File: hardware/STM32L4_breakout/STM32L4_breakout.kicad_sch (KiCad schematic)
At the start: 64 parts, among them J1 12V IN, J10 GPIO, J11 SPI1, J12 USART1, J13 USART3, J14 UART4, J15 3.3V, J16 5V, J17 12V, J2 SWD, J3 Conn_01x08, J4 Conn_01x06, J5 Conn_01x10, J6 Conn_01x08, J7 I2C1, J8 I2C2, J9 I2C3, SW1 SW_SPDT, U1 LD1117S50TR_SOT223, U2 LD3985M33R_SOT23, U3 LD1117S33TR_SOT223, U4 STM32L476RGTx, X1 NX3215SA-32.768K

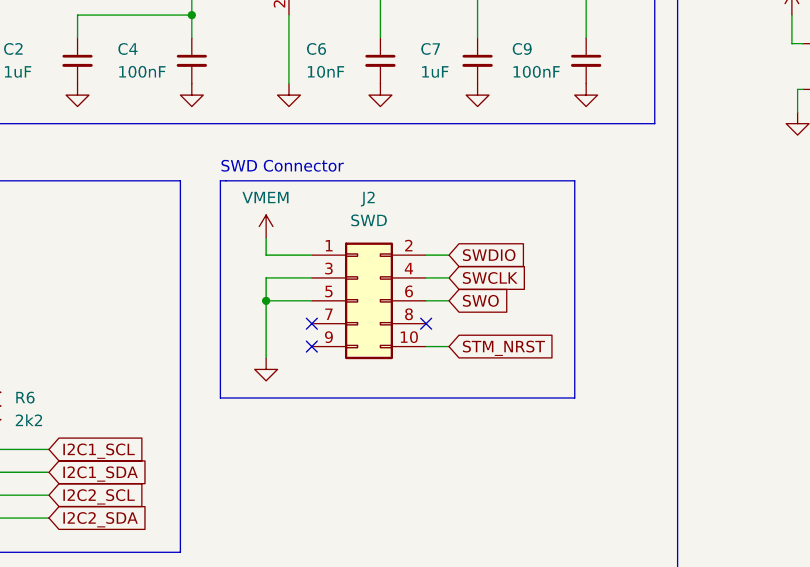
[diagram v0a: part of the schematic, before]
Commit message: breakout board PCB layout WIP
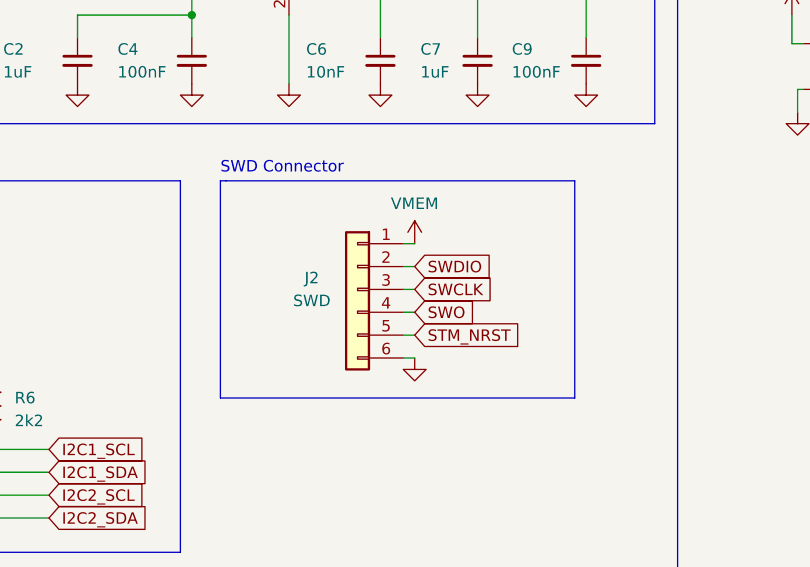
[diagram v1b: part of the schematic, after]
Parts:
- removed J2: SWD, Connector_PinHeader_2.54mm:PinHeader_2x05_P2.54mm_Vertical, symbol Connector_Generic:Conn_02x05_Odd_Even
- added J2: SWD, Connector_PinHeader_2.54mm:PinHeader_1x06_P2.54mm_Vertical, symbol Connector_Generic:Conn_01x06
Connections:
- net GND: now also J2.6 (Pin_6)
- net STM_NRST: now also J2.5 (Pin_5)
- net SWCLK: now also J2.3 (Pin_3)
- net SWDIO: now also J2.2 (Pin_2)
- net SWO: now also J2.4 (Pin_4)
- net VMEM: now also J2.1 (Pin_1)
- no-connect marks 33 -> 30

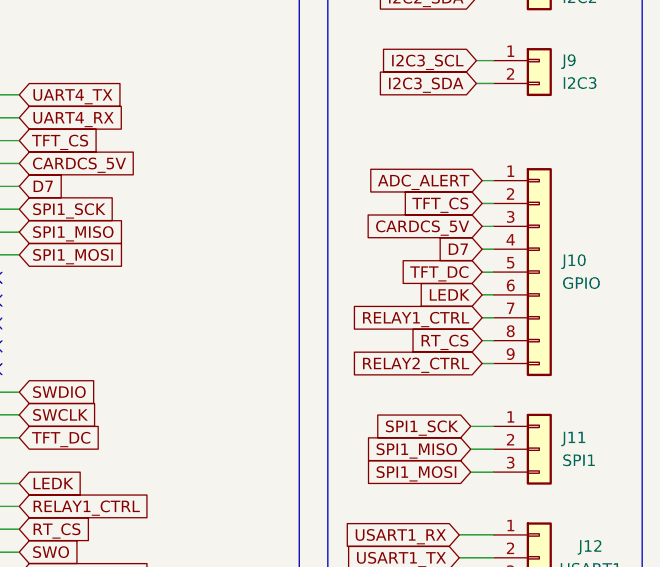
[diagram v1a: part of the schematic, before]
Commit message: breakout board PCB layout WIP
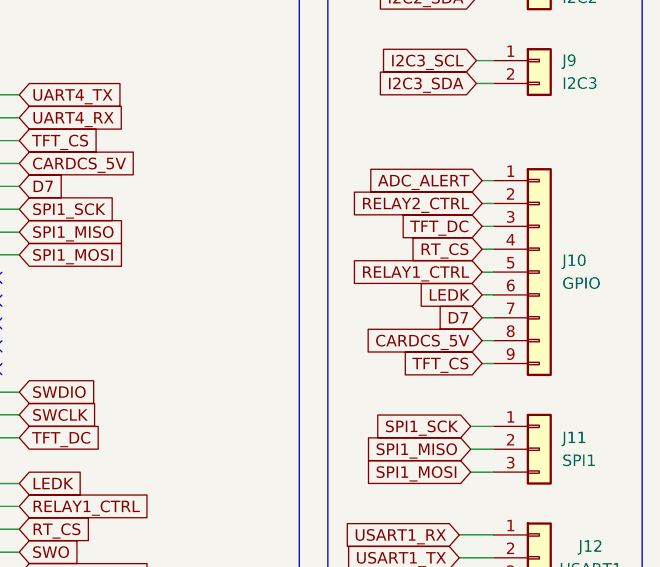
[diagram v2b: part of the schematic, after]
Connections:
- net CARDCS_5V: now also J10.8 (Pin_8); no longer J10.3 (Pin_3)
- net D7: now also J10.7 (Pin_7); no longer J10.4 (Pin_4)
- net RELAY1_CTRL: now also J10.5 (Pin_5); no longer J10.7 (Pin_7)
- net RELAY2_CTRL: now also J10.2 (Pin_2); no longer J10.9 (Pin_9)
- net RT_CS: now also J10.4 (Pin_4); no longer J10.8 (Pin_8)
- net TFT_CS: now also J10.9 (Pin_9); no longer J10.2 (Pin_2)
- net TFT_DC: now also J10.3 (Pin_3); no longer J10.5 (Pin_5)

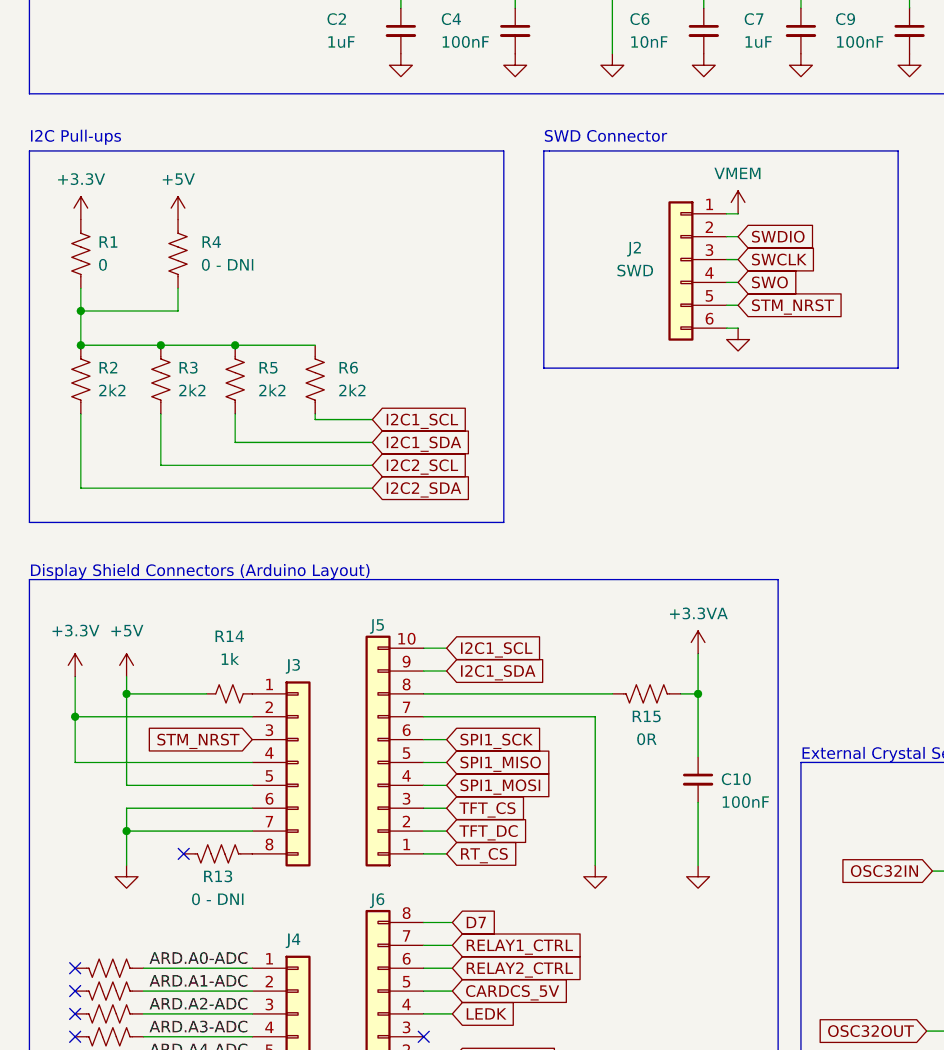
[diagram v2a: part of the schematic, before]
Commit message: breakout board layout WIP
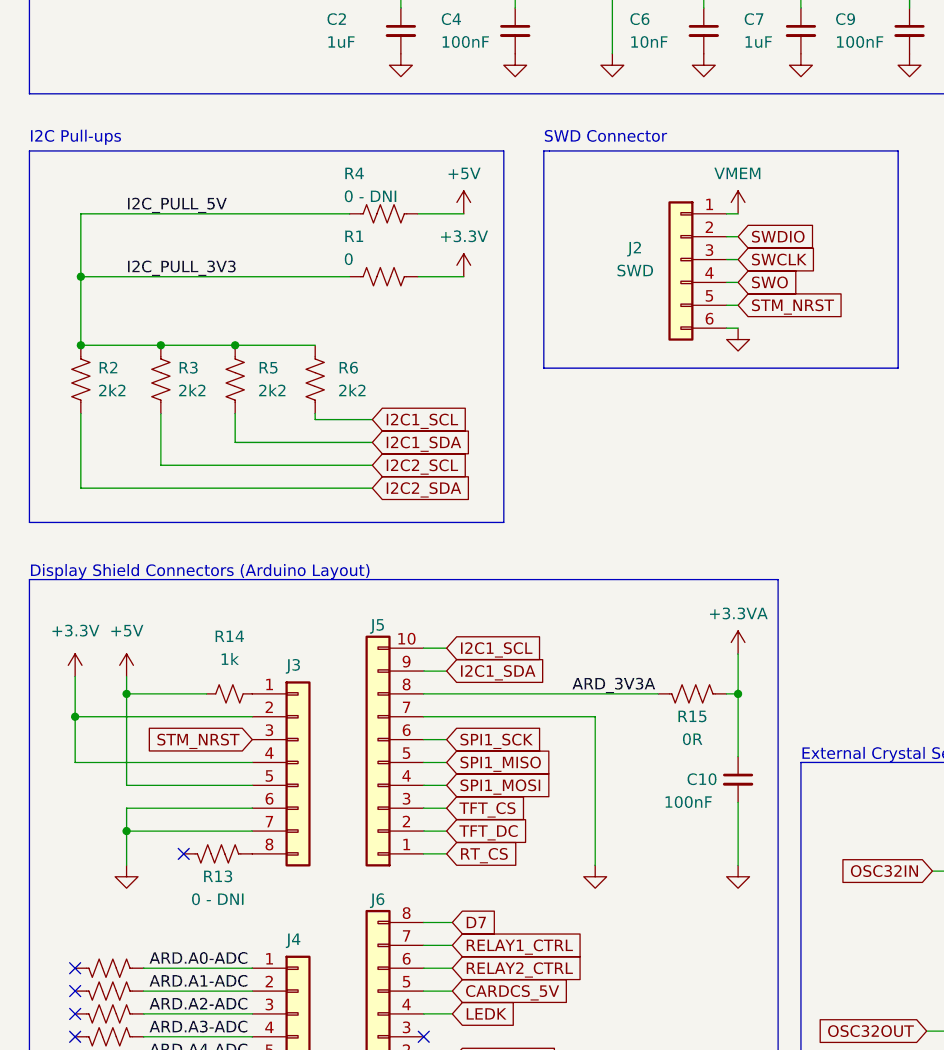
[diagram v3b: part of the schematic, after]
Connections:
- net I2C_PULL_3V3: now reaches R1.2, R2.1, R3.1, R4.2, R5.1, R6.1
- net ARD_3V3A: now reaches J5.8 (Pin_8), R15.2
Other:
- moved on the sheet: C10, R1, R15, R4
